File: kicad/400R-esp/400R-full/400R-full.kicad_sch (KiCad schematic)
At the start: 9 parts

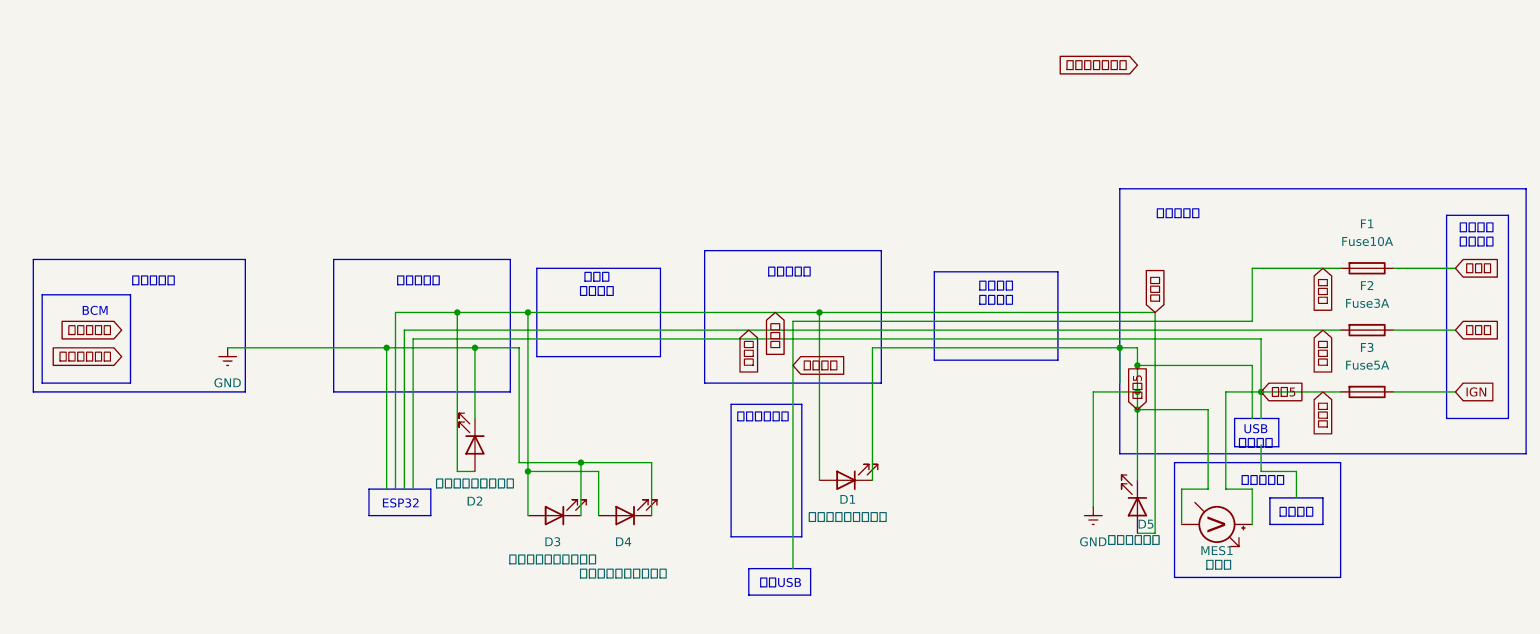
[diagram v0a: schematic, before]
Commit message: ハートライトの実装
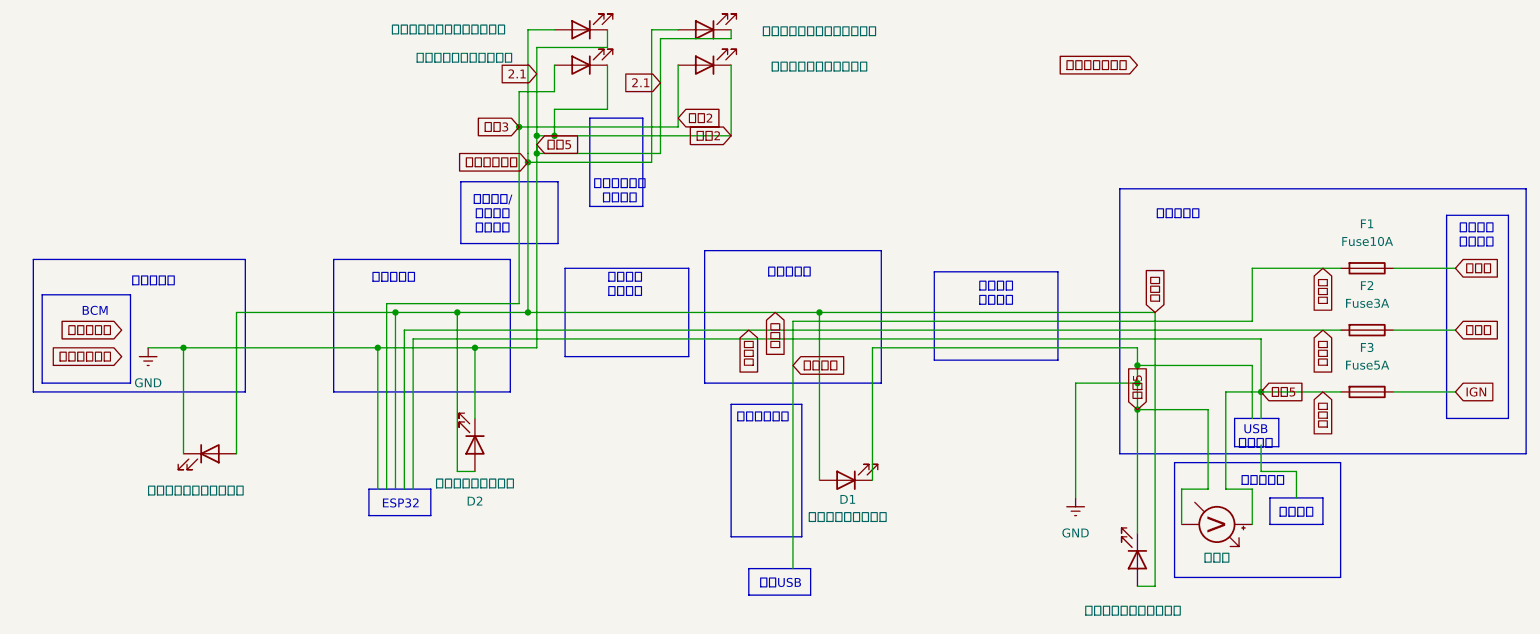
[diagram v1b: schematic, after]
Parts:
- added D6: エアコンハート運転席側, symbol Device:LED
- added D7: エアコンハート助手席側, symbol Device:LED
- added D8: エアコン間接助手席左側, symbol Device:LED
- D3: value エアコン間接助手席側 -> エアコン間接ナビ横助手席側
- D4: value エアコン間接運転席側 -> エアコン間接ナビ横運転席側
- D5: value エアコン間接 -> エアコン間接運転席右側
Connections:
- net GND: now also D6.1 (K), D6.2 (A), D7.1 (K), D7.2 (A), D8.1 (K), D8.2 (A)
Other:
- note added: "エアコン/ ナビ行き チューブ"
- note added: "ナビ上画面裏 チューブ"
- note added: "ナビ奥裏 チューブ"
- note removed: "ナビ裏 チューブ"
